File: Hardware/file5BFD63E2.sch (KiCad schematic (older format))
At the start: 8 parts, among them J18 Power_Connector_IO, J20 Digital_Connector_IO, J21 CV_Connector_IO, J22 Pot_Connector_IO, J23 Attenuverter_Connector_IO, J28 SID_Audio_Connector_IO

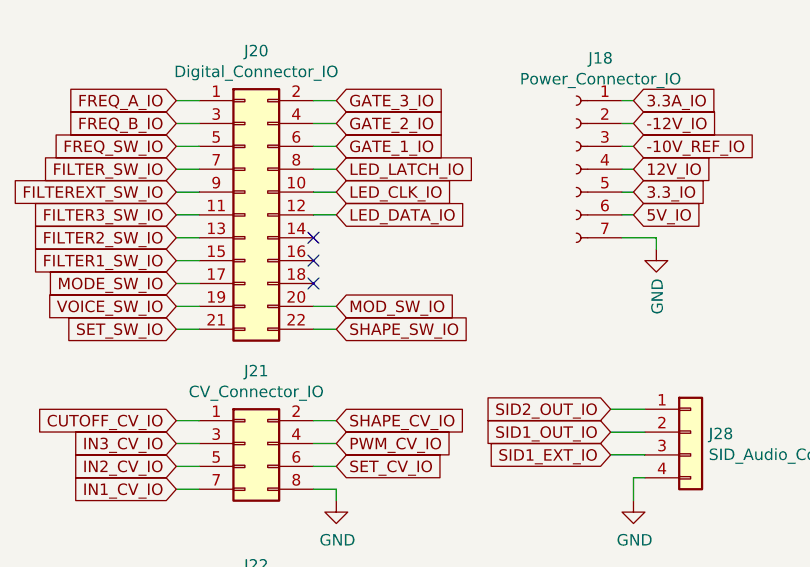
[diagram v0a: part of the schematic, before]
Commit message: Fixes #10
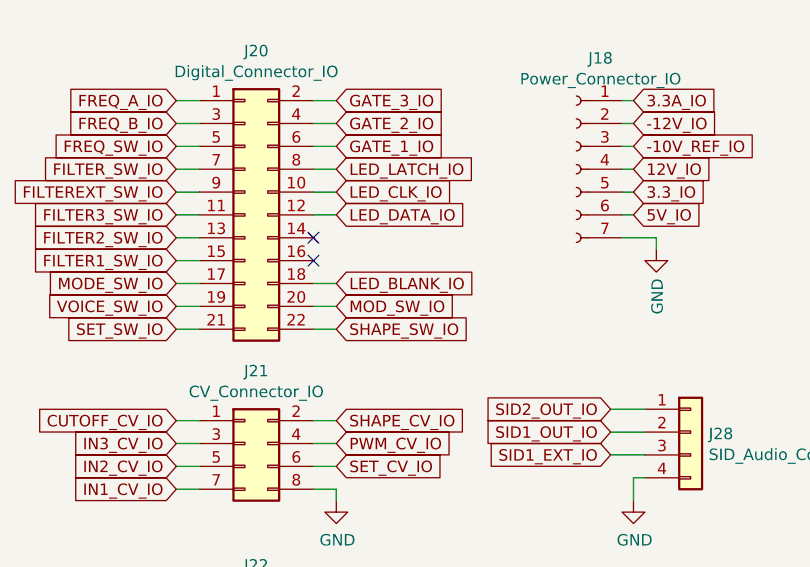
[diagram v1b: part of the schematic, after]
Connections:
- net LED_BLANK_IO: now reaches J20.18 (Pin_18)
- no-connect marks 3 -> 2
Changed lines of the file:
@@
 NoConn ~ 2350 3900
 NoConn ~ 2350 4000
-NoConn ~ 2350 4100
+Text GLabel 2450 4100 2    50   Input ~ 0
+LED_BLANK_IO
+Wire Wire Line
+	2450 4100 2350 4100
 $EndSCHEMATC
